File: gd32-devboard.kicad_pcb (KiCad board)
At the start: 4 copper layers, 49.8 x 80.1 mm, 102 parts, among them J201 Conn_02x05_Odd_Even, J202 J_TC2030-IDC, J301 J_TC2030-IDC, J401 DB9_Female_MountingHoles, J601 J_USB_B_Mini, J701 J_Micro_SD_Card, J801 SPI, J901 Conn_02x05_Counter_Clockwise, Q301 Q_SOT23_NPN, Q302 Q_SOT23_NPN, U201 U_GD32F405RGT6, U301 U_ATGM336H-5N31, U302 U_ESP32-C3-MINI-1U-N4, U303 U_AT2659, U304 U_RA-01S, U401 U_LM317_TO-252, U402 U_TLV61046ADB, U501 U_TJA1050, U601 U_TS3USB30ERSWR, Y201 Y_32.768k, Y202 Y_8m

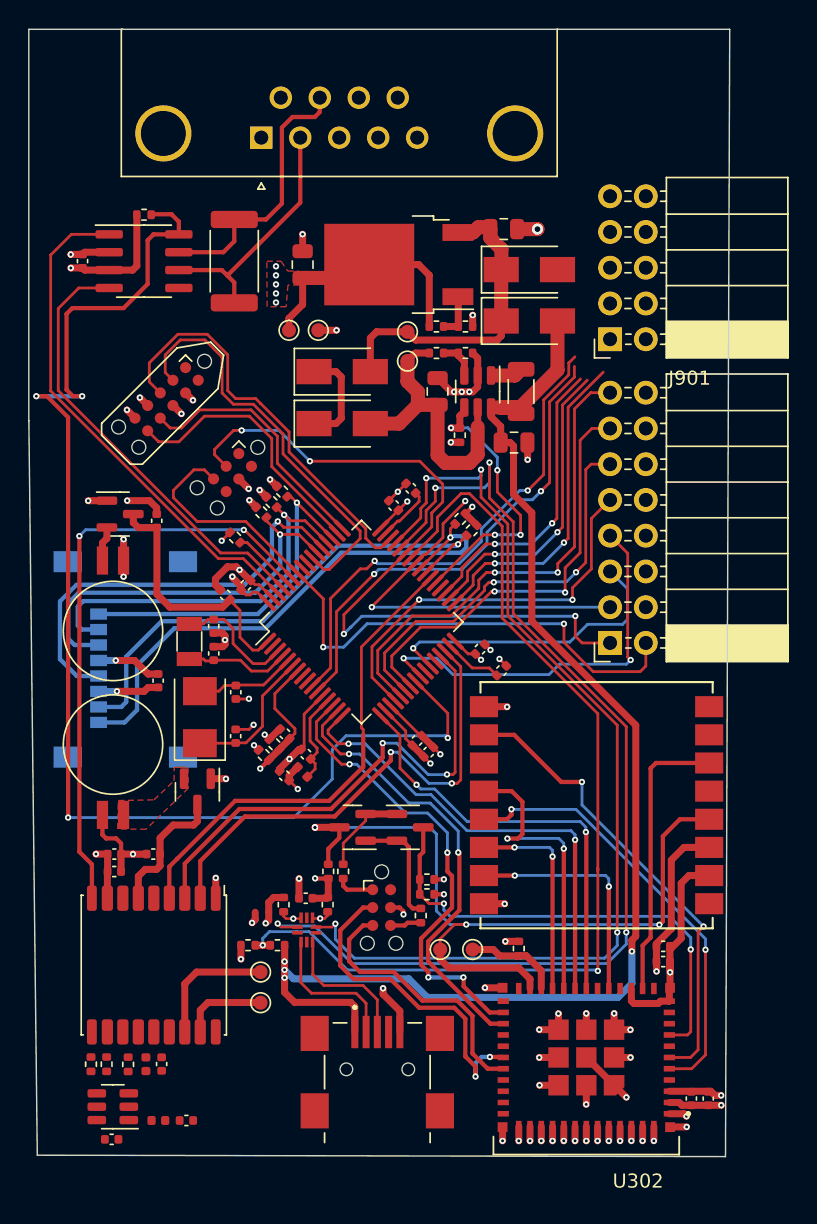
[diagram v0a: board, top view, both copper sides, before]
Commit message: layout: progress
Signed-off-by: Connor Rigby <connorr@hey.com>
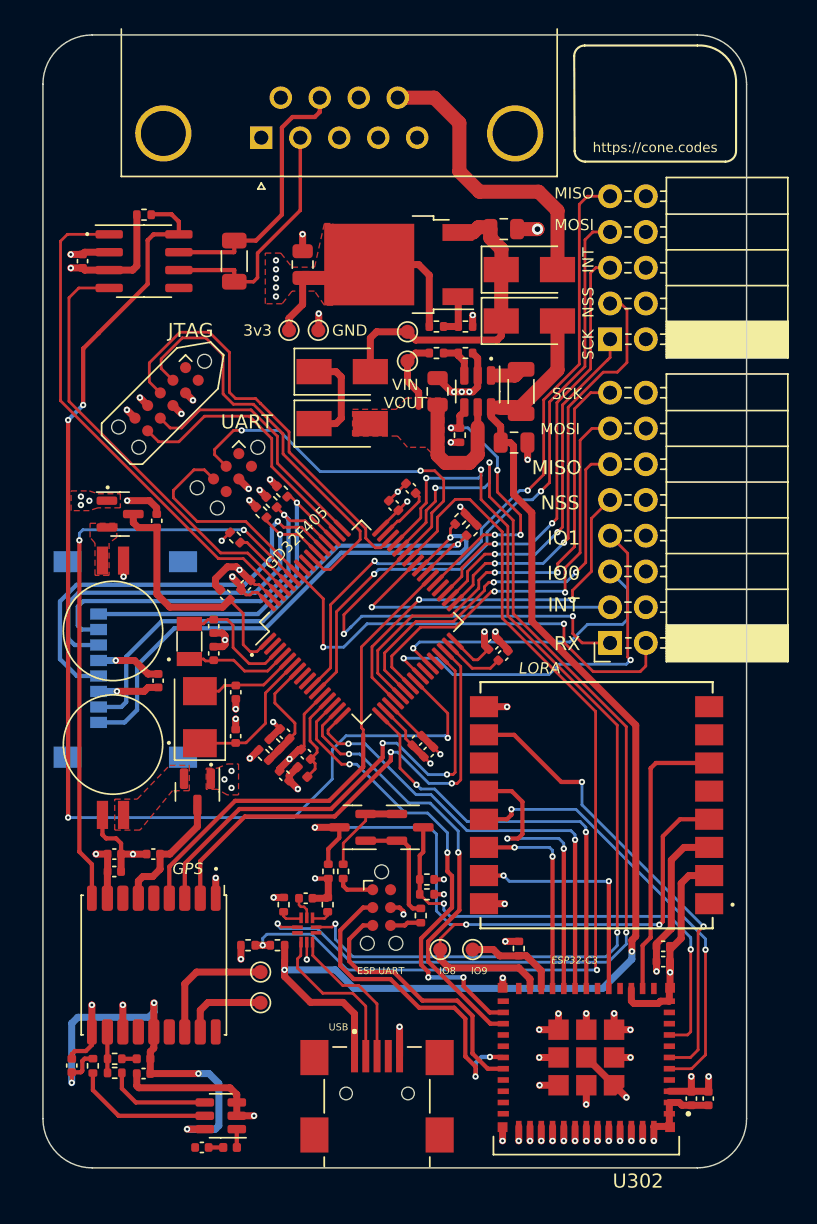
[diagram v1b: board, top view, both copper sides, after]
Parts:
- C305: value C_0402_DNP -> C_0402_470p
- FB201: value FerriteBead_Small -> FB_0402_1k
- J801: value SPI -> SPI1
- J901: value Conn_02x05_Counter_Clockwise -> SPI2
- L301: value L_0402_DNP -> L_6n8
- R502: value R_120_2512 -> R_120_1206; footprint Resistor_SMD:R_2512_6332Metric -> Resistor_SMD:R_1206_3216Metric
- moved U303 7.70 mm to (30.6, 104.8)
- moved C307 5.96 mm to (20.1, 101.2), turned to 90 degrees
- moved L301 5.44 mm to (31.3, 107.0), turned to 180 degrees
- moved C305 2.21 mm to (29.3, 107.0), turned to 180 degrees
- moved J601 1.71 mm to (41.7, 103.2)
- moved C304 1.45 mm to (25.1, 101.8), turned to 180 degrees
- moved C206 1.07 mm to (50.7, 72.1)
- moved R308 1.03 mm to (23.1, 100.8), turned to 0 degrees
- moved C212 1.00 mm to (50.0, 71.3)
- moved R307 0.84 mm to (23.1, 101.8), turned to 0 degrees
- moved L302 0.42 mm to (25.1, 100.8), turned to 180 degrees
- moved R309 0.18 mm to (21.6, 101.2)
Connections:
- net /Wireless/RF_IN renamed /Wireless/LNA_RF_IN
- C601 pad 1: +3V3 -> /USB/USB_ESD_VCC
- J901 pad 1: /Base/SPI2_INT -> /Base/SPI2_SCK
- J901 pad 3: /Base/SPI2_SCK -> /Base/SPI2_NSS
- J901 pad 5: /Base/SPI2_NSS -> /Base/SPI2_INT
- J901 pad 7: /Base/SPI2_MISO -> /Base/SPI2_MOSI
- J901 pad 9: /Base/SPI2_MOSI -> /Base/SPI2_MISO
- U601 pad 4: GND -> /USB/USB_ESD_GND
- U601 pad 9: +3V3 -> /USB/USB_ESD_VCC
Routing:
- net /Wireless/VCC_RF: track 0.00 -> 31.0 mm, vias 0 -> 4
- net /Power/12VIN: track 0.00 -> 20.9 mm
- net /Base/SPI2_MISO: track 35.5 -> 48.6 mm
- net /Base/SPI2_MOSI: track 34.6 -> 46.0 mm
- net GND: track 133.8 -> 144.9 mm, vias 69 -> 67
- net /Wireless/~{GPS_RF_SHDN}: track 0.00 -> 9.92 mm
- net /Base/SPI2_INT: track 21.1 -> 30.5 mm
- net /Base/CAN_STBY: track 92.2 -> 84.5 mm
- net Net-(R307-Pad2): track 0.00 -> 7.41 mm
- net /Base/SPI2_NSS: track 23.2 -> 30.3 mm
- net /Base/SPI1_INT: track 27.3 -> 21.3 mm, vias 2 -> 1
- net /Power/VOUT: track 20.8 -> 15.6 mm
- net /Base/SPI2_SCK: track 21.6 -> 25.2 mm
- net /Wireless/GPS_RF_IN: track 0.00 -> 2.91 mm
- net +3V3: track 76.5 -> 73.6 mm, vias 26 -> 29
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- added copper zone on In1.Cu, net +3V3
- added copper zone on F.Cu, net /Power/VOUT
- added copper zone on F.Cu, net Net-(BT201-Pad1)
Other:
- board size 49.8 x 80.1 mm -> 50 x 80.5 mm
- board text added: "3v3"
- board text added: "ESP UART"
- board text added: "ESP32-C3"
- board text added: "GD32F405"
- board text added: "GND"
- board text added: "GPS"
- board text added: "INT"
- board text added: "IO0"
- board text added: "IO1"
- board text added: "IO8"
- board text added: "IO9"
- board text added: "JTAG"
- board text added: "LORA"
- board text added: "MISO"
- board text added: "MOSI"
- board text added: "NSS"
- board text added: "RX"
- board text added: "SCK"
- board text added: "UART"
- board text added: "USB"
- board text added: "VIN VOUT"
- board text added: "https://cone.codes"
